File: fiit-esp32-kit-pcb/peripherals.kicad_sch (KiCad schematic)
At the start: 21 parts, among them Q2 SFH320, SW1 SPST NO, SW2 SPST NO, SW3 SPST NO, SW4 SPST NO, U4 AHT20

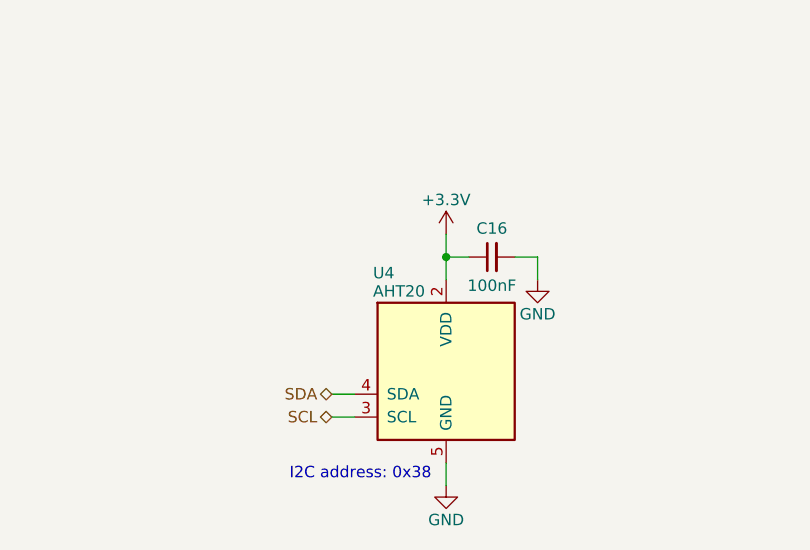
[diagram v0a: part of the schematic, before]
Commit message: footprints assignment
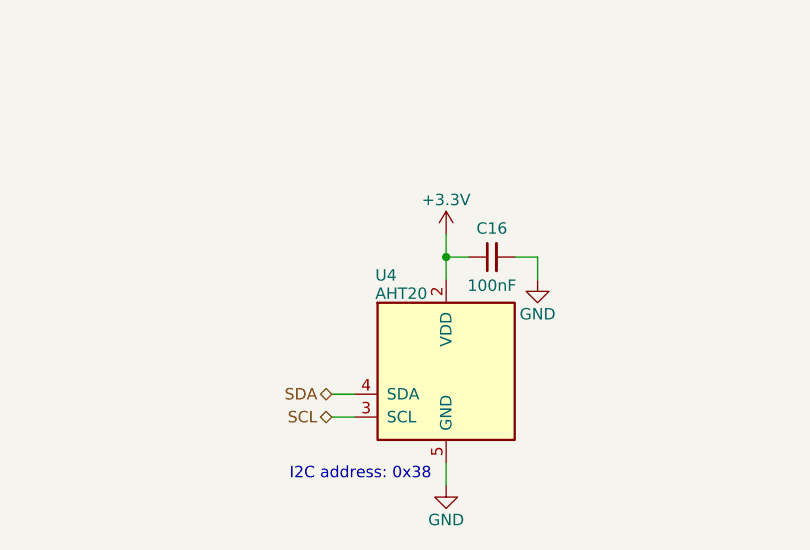
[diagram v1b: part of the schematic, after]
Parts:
- removed U4: AHT20, Findemm:AHT20, symbol Findemm:AHT20
- added U4: AHT20, FIIT_Kit:AHT20, symbol FIIT_Kit:AHT20
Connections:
- net +3.3V: now also U4.2 (VDD)
- net GND: now also U4.5 (GND)
- net SCL: now also U4.3 (SCL)
- net SDA: now also U4.4 (SDA)
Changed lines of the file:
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@@
+	)
+	(symbol
+		(lib_id "FIIT_Kit:AHT20")
+		(at 101.6 132.08 0)
+		(unit 1)
+		(exclude_from_sim no)
+		(in_bom yes)
+		(on_board yes)
+		(dnp no)
+		(property "Reference" "U4"
+			(at 93.726 121.412 0)
+			(effects
+				(font
+					(size 1.27 1.27)
+				)
+				(justify left)
+			)
+		)
+		(property "Value" "AHT20"
+			(at 93.726 123.444 0)
+			(effects
+				(font
+					(size 1.27 1.27)
+				)
+				(justify left)
+			)
+		)
+		(property "Footprint" "FIIT_Kit:AHT20"
+			(at 101.6 132.08 0)
+			(effects
+				(font
+					(size 1.27 1.27)
+				)
+				(justify bottom)
+				(hide yes)
+			)
+		)
+		(property "Datasheet" "https://files.seeedstudio.com/wiki/Grove-AHT20_I2C_Industrial_Grade_Temperature_and_Humidity_Sensor/AHT20-datasheet-2020-4-16.pdf"
+			(at 101.6 132.08 0)
+			(effects
+				(font
+					(size 1.27 1.27)
+				)
+				(hide yes)
+			)
+		)
+		(property "Description" ""
+			(at 101.6 132.08 0)
+			(effects
+				(font
+					(size 1.27 1.27)
+				)
+				(hide yes)
+			)
+		)
+		(property "LCSC" "C2757850"
+			(at 101.6 132.08 0)
+			(effects
+				(font
+					(size 1.27 1.27)
+				)
+				(hide yes)
+			)
+		)
+		(property "Manufacturer Part Number" "AHT20"
+			(at 101.6 132.08 0)
+			(effects
+				(font
+					(size 1.27 1.27)
+				)
+				(hide yes)
+			)
+		)
+		(pin "4"
+		)
+		(pin "3"
+		)
+		(pin "1"
+		)
+		(pin "2"
+		)
+		(pin "5"
+		)
+		(pin "6"
+		)
+		(instances
+			(project ""
+				(path "/d7013812-ce13-4db9-a6cc-42acdc5acaf9/fe4defb8-cb63-4770-8d91-1c7f8da70e07"
+					(reference "U4")
+					(unit 1)
+				)
+			)
+		)
 	)
 	(symbol
@@
 					(unit 1)
 				)
-			)
-		)
-	)
-	(symbol
-		(lib_id "Findemm:AHT20")
-		(at 101.6 132.08 0)
-		(unit 1)
-		(exclude_from_sim no)
-		(in_bom yes)
-		(on_board yes)
-		(dnp no)
-		(property "Reference" "U4"
-			(at 93.472 121.158 0)
-			(effects
-				(font
-					(size 1.27 1.27)
-				)
-				(justify left)
-			)
-		)
-		(property "Value" "AHT20"
-			(at 93.472 123.19 0)
-			(effects
-				(font
-					(size 1.27 1.27)
-				)
-				(justify left)
-			)
-		)
-		(property "Footprint" "Findemm:AHT20"
-			(at 101.6 132.08 0)
-			(effects
-				(font
-					(size 1.27 1.27)
-				)
-				(justify bottom)
-				(hide yes)
-			)
-		)
-		(property "Datasheet" "https://files.seeedstudio.com/wiki/Grove-AHT20_I2C_Industrial_Grade_Temperature_and_Humidity_Sensor/AHT20-datasheet-2020-4-16.pdf"
-			(at 101.6 132.08 0)
-			(effects
-				(font
-					(size 1.27 1.27)
-				)
-				(hide yes)
-			)
-		)
-		(property "Description" ""
-			(at 101.6 132.08 0)
-			(effects
-				(font
-					(size 1.27 1.27)
-				)
-				(hide yes)
-			)
-		)
-		(property "LCSC" "C2757850"
-			(at 101.6 132.08 0)
-			(effects
-				(font
-					(size 1.27 1.27)
-				)
-				(hide yes)
-			)
-		)
-		(property "Manufacturer Part Number" "AHT20"
-			(at 101.6 132.08 0)
-			(effects
-				(font
-					(size 1.27 1.27)
-				)
-				(hide yes)
-			)
-		)
-		(pin "2"
-		)
-		(pin "3"
-		)
-		(pin "4"
-		)
-		(pin "5"
-		)
-		(pin "1"
-		)
-		(pin "6"
-		)
-		(instances
-			(project "fiit-esp32-kit-pcb"
-				(path "/d7013812-ce13-4db9-a6cc-42acdc5acaf9/fe4defb8-cb63-4770-8d91-1c7f8da70e07"
-					(reference "U4")
-					(unit 1)
-				)
